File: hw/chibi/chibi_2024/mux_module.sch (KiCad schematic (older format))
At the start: 6 parts

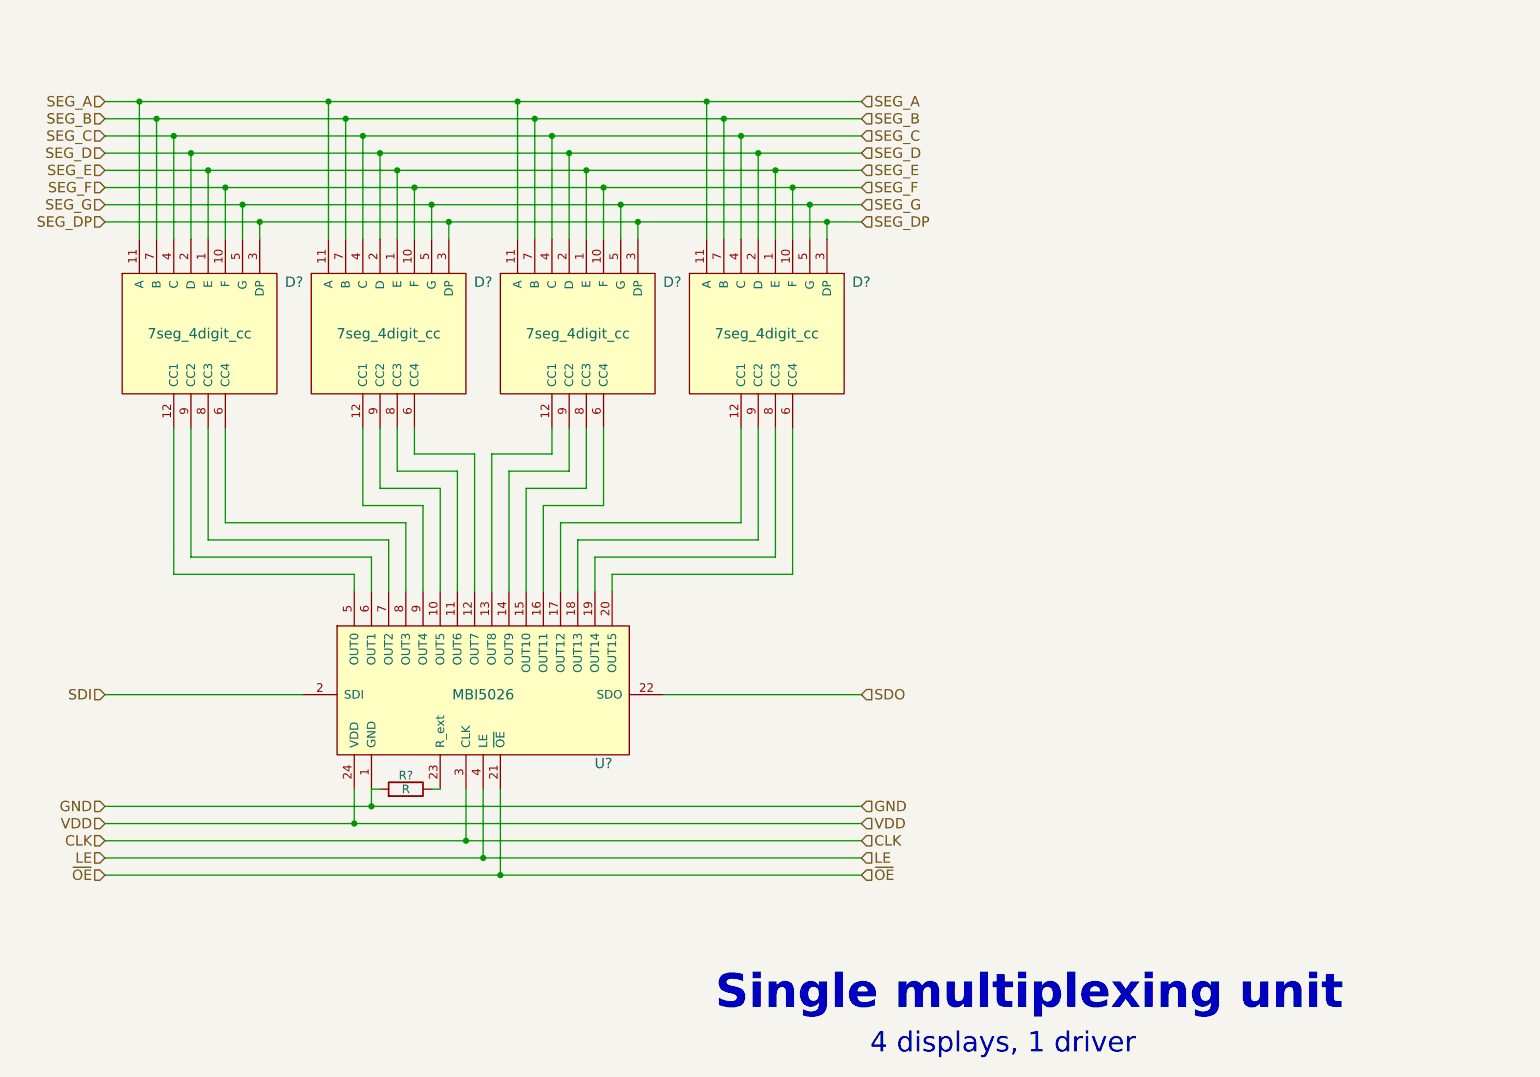
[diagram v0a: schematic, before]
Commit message: Added protection stuff
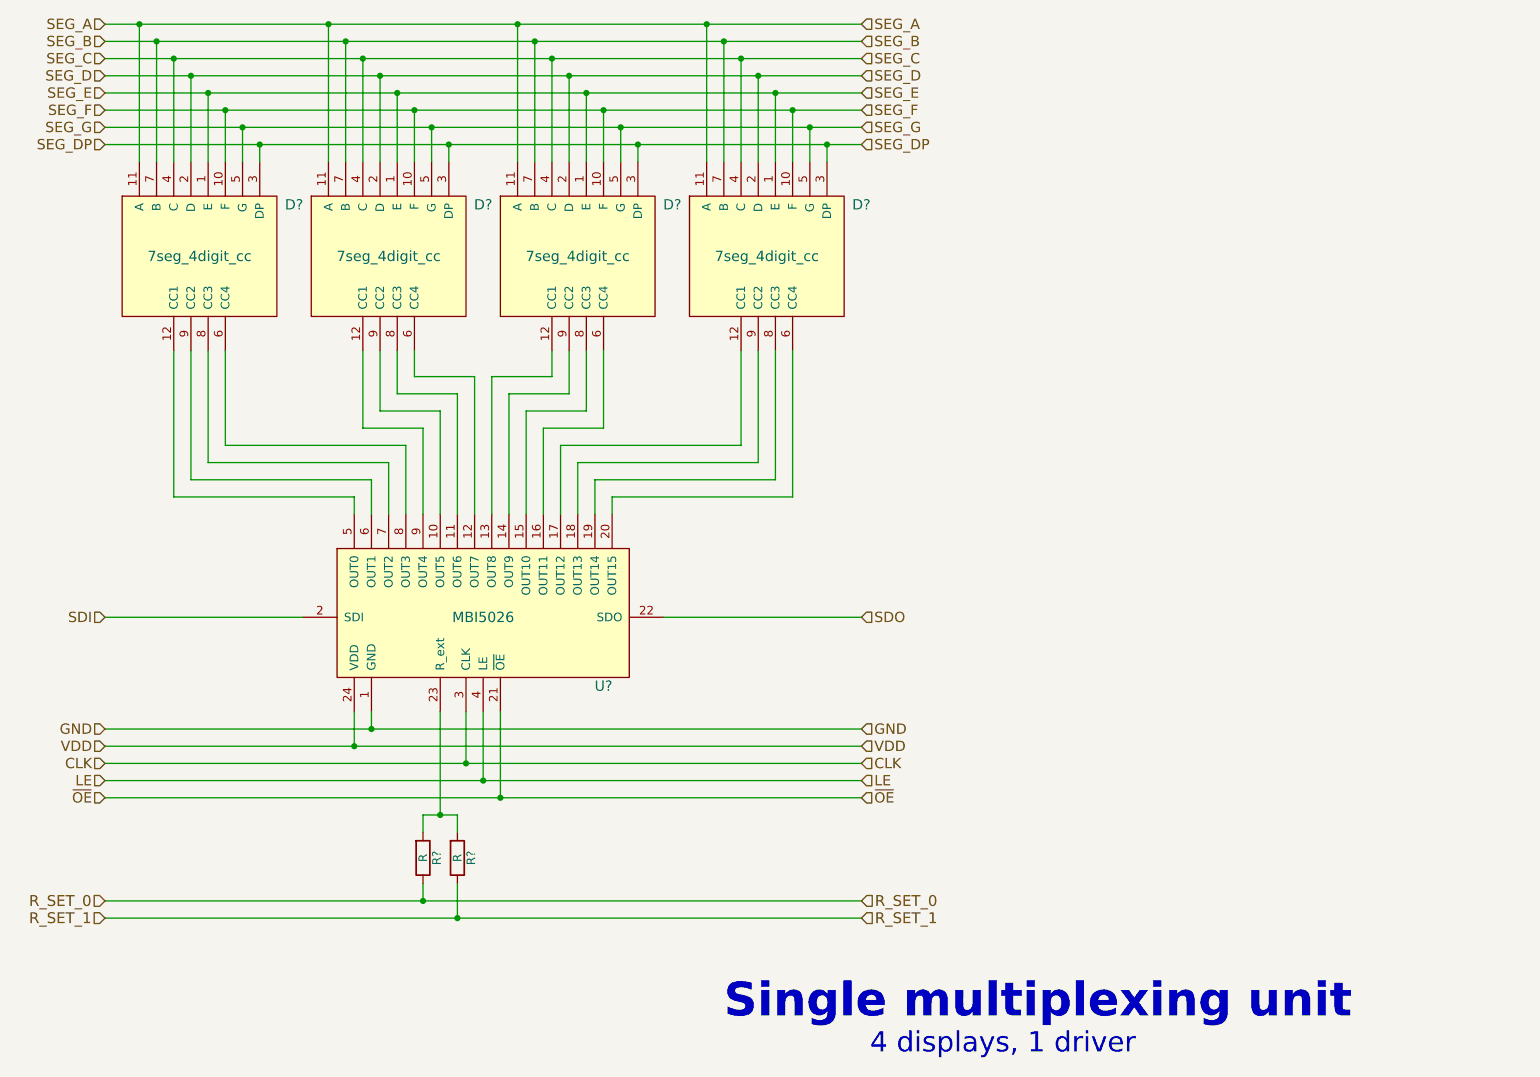
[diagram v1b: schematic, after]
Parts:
- added R?: R, symbol R
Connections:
- net GND: no longer R?.2
- net at U?.23 (R_ext): now also R?.2, R?.2; no longer R?.1
- new net R_SET_0: R?.1
- new net R_SET_1: R?.1
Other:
- moved on the sheet: D?, R?, U?
